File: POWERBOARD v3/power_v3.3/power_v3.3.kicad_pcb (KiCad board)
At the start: 4 copper layers, 60 x 34.1 mm, 63 parts, among them IC1 MAX25301AATB_V+T, IC2 MCP6541T-I_OT, IC3 AP2281-1FMG-7, J1 43650-0300, J2 UJ20-C-H-G-SMT-1-P16-TR, J3 2053380002, U1 USBLC6-2, U2 BQ25886RGE, U3 TPS62160DSG

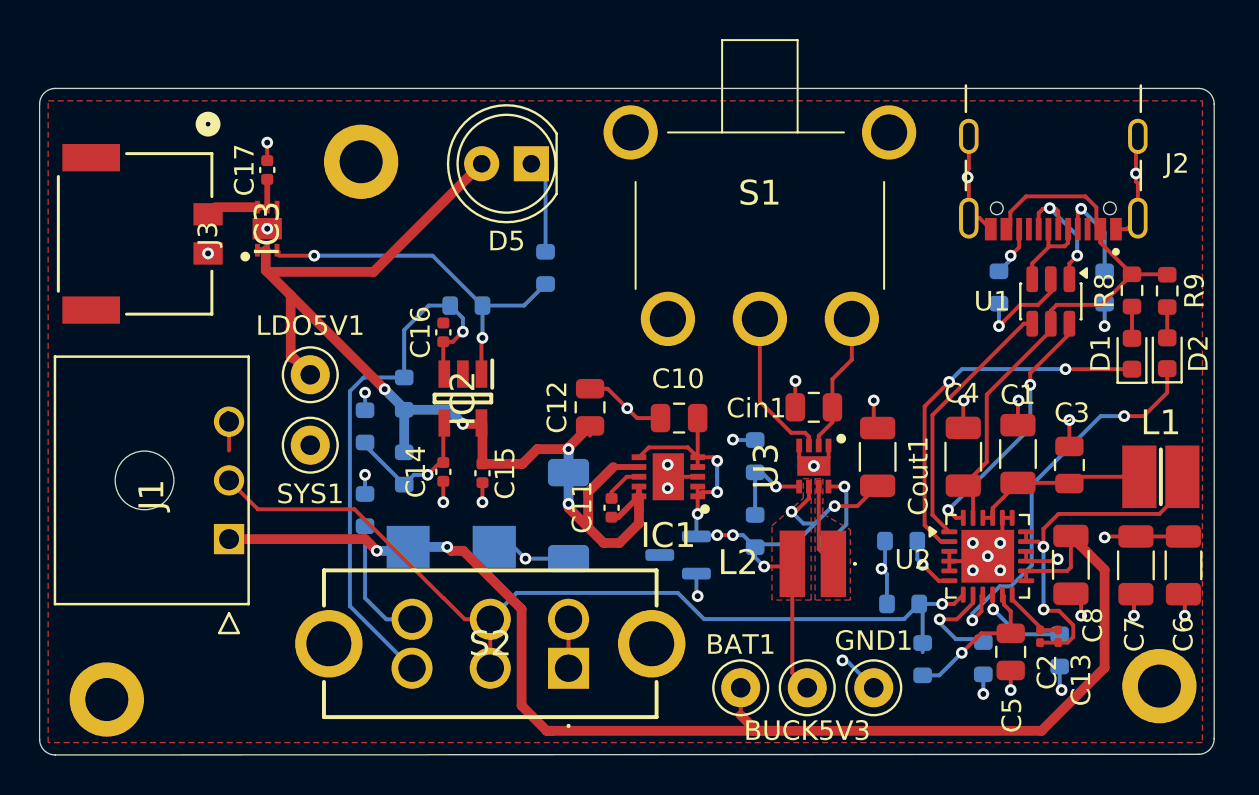
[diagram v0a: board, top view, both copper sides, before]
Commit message: Update PowerBoard
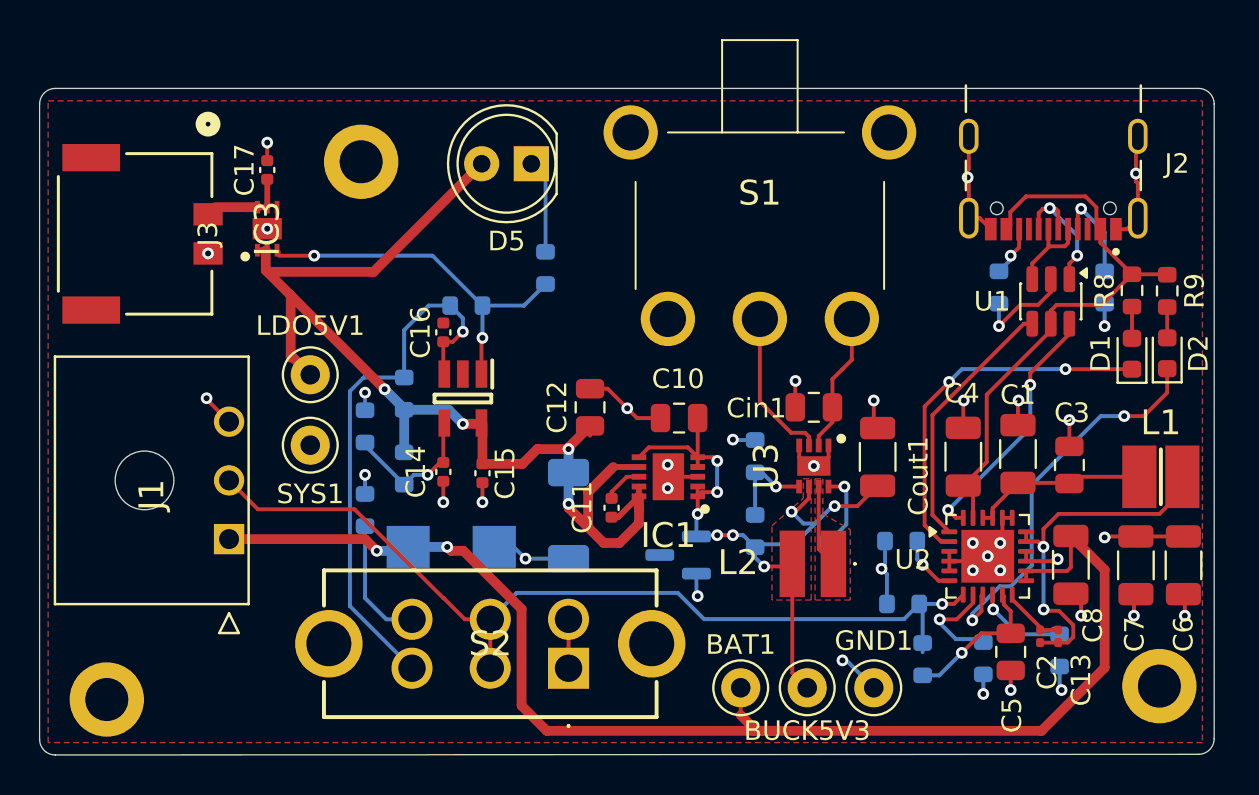
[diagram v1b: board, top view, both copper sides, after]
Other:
- board text added: "Power Board"
